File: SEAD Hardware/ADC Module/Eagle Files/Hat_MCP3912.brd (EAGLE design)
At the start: 45 x 36.5 mm, 36 parts, among them IC1 MCP3912, X2 52885-0374

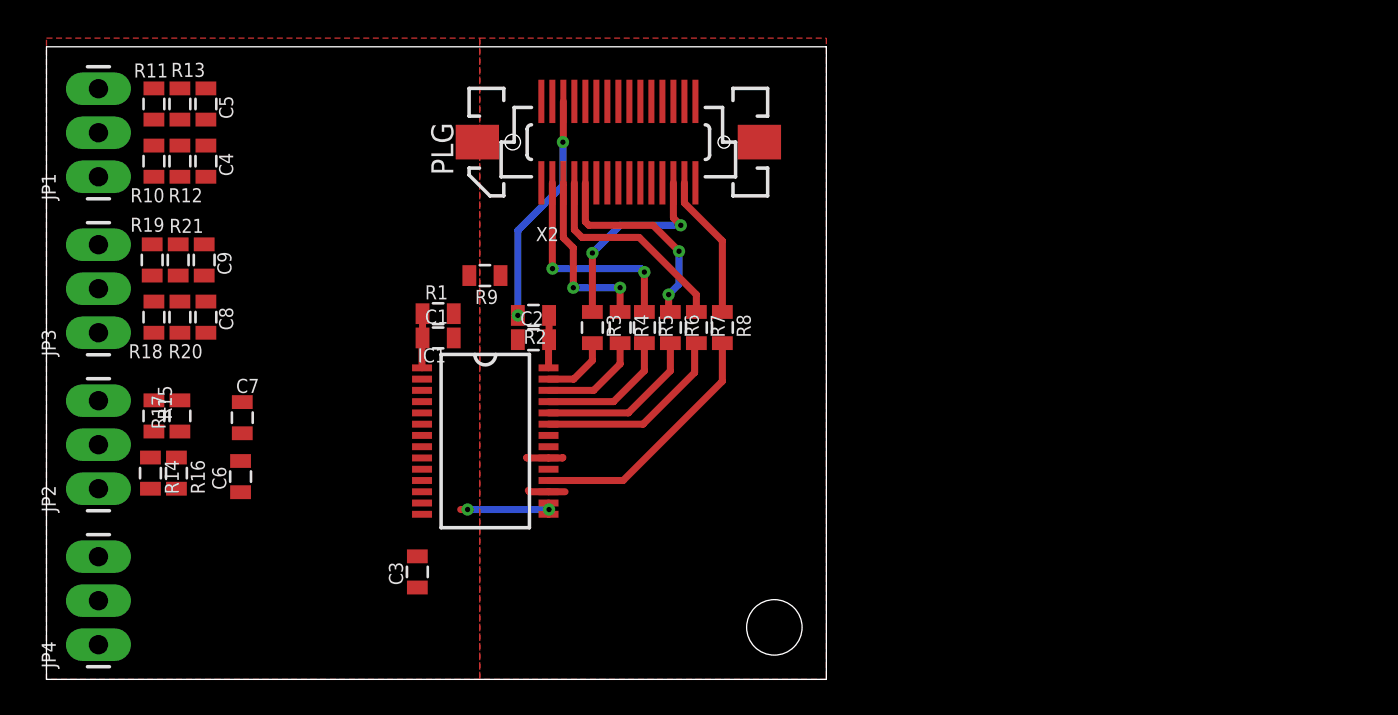
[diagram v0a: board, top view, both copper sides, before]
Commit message: More board work.
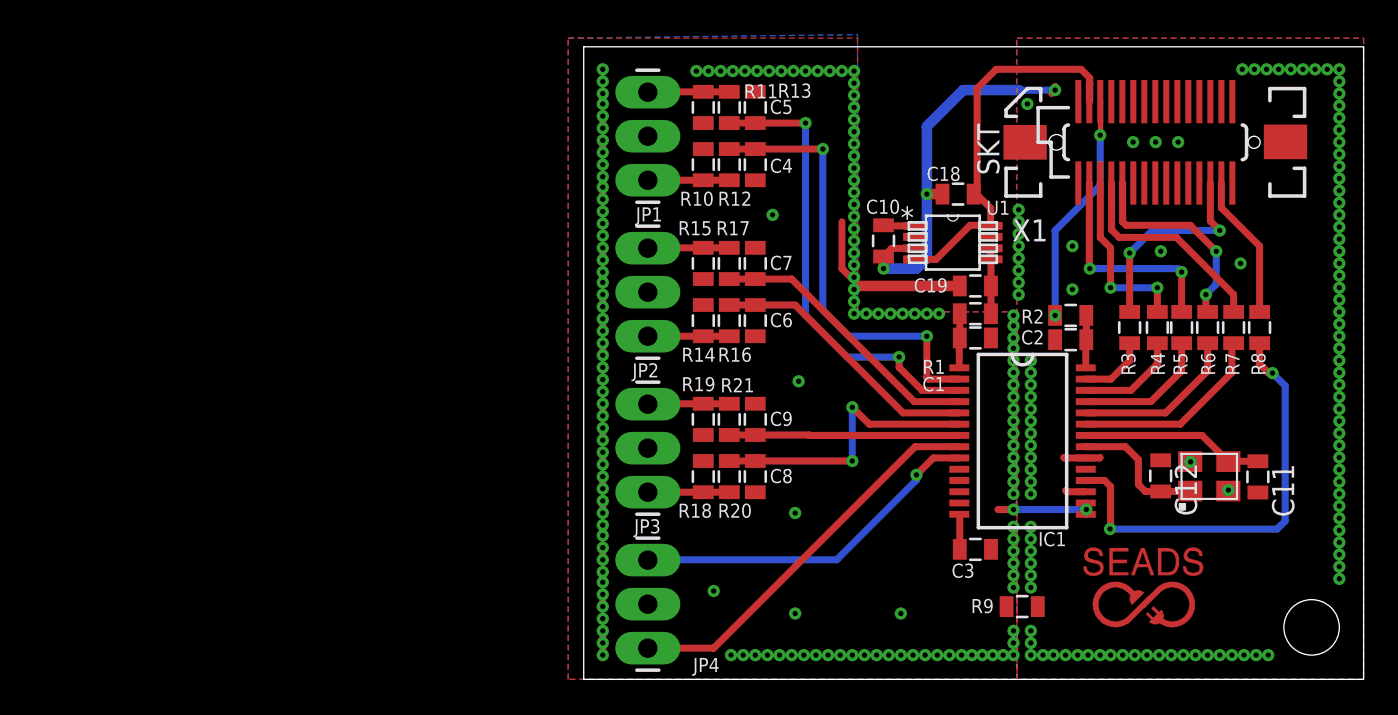
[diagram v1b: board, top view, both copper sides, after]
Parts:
- removed X2: 52885-0374, SensorCape:52885-0374
- added C10: .01uF, SensorCape:0805
- added C11, C12: 20pF, SensorCape:0805
- added C18: 2.2uF, SensorCape:0805
- added C19: 4.7uF, SensorCape:0805
- added U$1: 7M-12.000MEEQ-T, SensorCape:7M-CRYSTAL
- added U1: LP2989_DGK_8, SensorCape:MUA08A
- added X1: 55091-0374, SensorCape:55091-0374
- moved R9 36.4 mm to (56.3, 4.20)
- moved C9 33.1 mm to (40.9, 15.0)
- moved R19 33.1 mm to (37.9, 15.0)
- moved R21 33.1 mm to (39.4, 15.0)
- moved R14 33.1 mm to (37.9, 20.7)
- moved R16 33.1 mm to (39.4, 20.7)
- moved JP3 33.0 mm to (34.7, 10.8)
- moved C8 33.0 mm to (40.9, 11.7)
- moved R18 33.0 mm to (37.9, 11.7)
- moved R20 33.0 mm to (39.4, 11.7)
- moved JP2 32.9 mm to (34.7, 19.8)
- moved R15 32.9 mm to (37.9, 24.0)
- moved R17 32.9 mm to (39.4, 24.0)
- moved C3 32.2 mm to (53.6, 7.50), turned to 180 degrees
- moved JP1 31.7 mm to (34.7, 28.8)
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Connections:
- new net N$24: C10.2, U1.1
- new net N$26: C11.1, IC1.22, U$1.3
- new net N$27: C12.2, IC1.21, U$1.1
- net AGND: now also C19.1, JP1.2, JP2.2, JP3.2, JP4.2
- net GND: now also C10.1, C11.2, C12.1, C18.2, U$1.2, U$1.4, U1.3, X1.1, X1.12, X1.18, X1.2, X1.24, X1.29, X1.30; no longer X2.1, X2.11, X2.17, X2.2, X2.23, X2.29, X2.30
- net MISO: now also X1.4; no longer X2.3
- net MOSI: now also X1.6; no longer X2.5
- net SCK: now also X1.10; no longer X2.9
- net SCL: now also X1.16; no longer X2.15
- net SDA: now also X1.14; no longer X2.13
- net SS: now also X1.8; no longer X2.7
- net U1RX: now also X1.22; no longer X2.21
- net U1TX: now also X1.20; no longer X2.19
- net U3RX: now also X1.28; no longer X2.27
- net U3TX: now also X1.26; no longer X2.25
- net VDD3V3_A: now also C19.2, U1.5, U1.6
- net VDD3V3_D: now also X1.5; no longer X2.6
- net VDD5V0_D: now also C18.1, U1.4, U1.8, X1.3; no longer X2.4
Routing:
- net N$14: track 0.00 -> 26.5 mm, vias 0 -> 2
- net N$13: track 0.00 -> 25.6 mm, vias 0 -> 2
- net VDD5V0_D: track 0.00 -> 23.2 mm
- net N$22: track 0.00 -> 22.8 mm
- net AGND: track 6.04 -> 28.4 mm, vias 2 -> 148
- net GND: track 4.28 -> 26.2 mm, vias 0 -> 113
- net N$23: track 0.00 -> 20.6 mm, vias 0 -> 1
- net N$20: track 0.00 -> 16.8 mm, vias 0 -> 2
- net N$17: track 0.00 -> 16.2 mm
- net N$16: track 0.00 -> 15.8 mm
- net N$21: track 0.00 -> 13.3 mm
- net N$7: track 14.6 -> 25.3 mm, vias 0 -> 2
- net N$26: track 0.00 -> 10.6 mm
- net N$27: track 0.00 -> 7.95 mm
- net N$19: track 0.00 -> 4.71 mm
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- added copper zone on layer 16, net AGND
- added copper zone on layer 16, net GND
